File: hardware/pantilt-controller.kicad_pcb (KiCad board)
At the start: 4 copper layers, 52.3 x 93.2 mm, 84 parts, among them J1 Conn_01x22_Socket, J17 Motor_Slide, J18 Motor_Pan, J19 Motor_Tilt, J2 Conn_01x22_Socket, J20 TCA9548A_Mux, J21 AS5600_Pan, J22 AS5600_Tilt, J23 OLED, J24 TCA9548A_Mux, J26 Limit_Min, J27 Limit_Max, J28 Motor_Aux, J29 Enc_Slide, J3 MUX_2, J30 Enc_Pan, J31 Enc_Tilt, J32 Enc_Aux, J33 Btn_SetKeyframe, J34 Btn_ClearKeyframe, J35 Btn_PlayPause, J36 Btn_Reset, J37 5V_In, J38 24V_In, J4 MUX_3, J41 Aux_Max, J5 MUX_4, J6 MUX_5, J7 MUX_6, J8 MUX_7, U1 tmc2209, U2 tmc2209, U3 tmc2209, U4 tmc2209

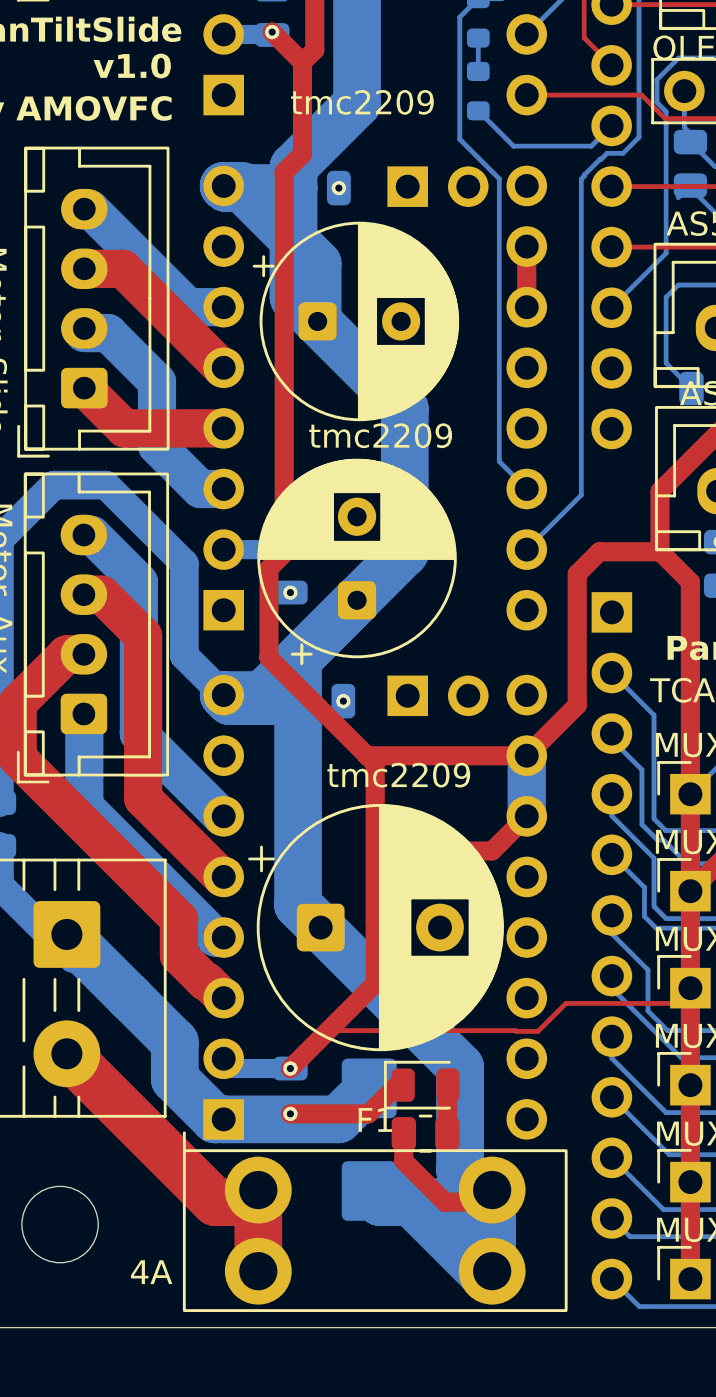
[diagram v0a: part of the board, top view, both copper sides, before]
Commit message: fixes
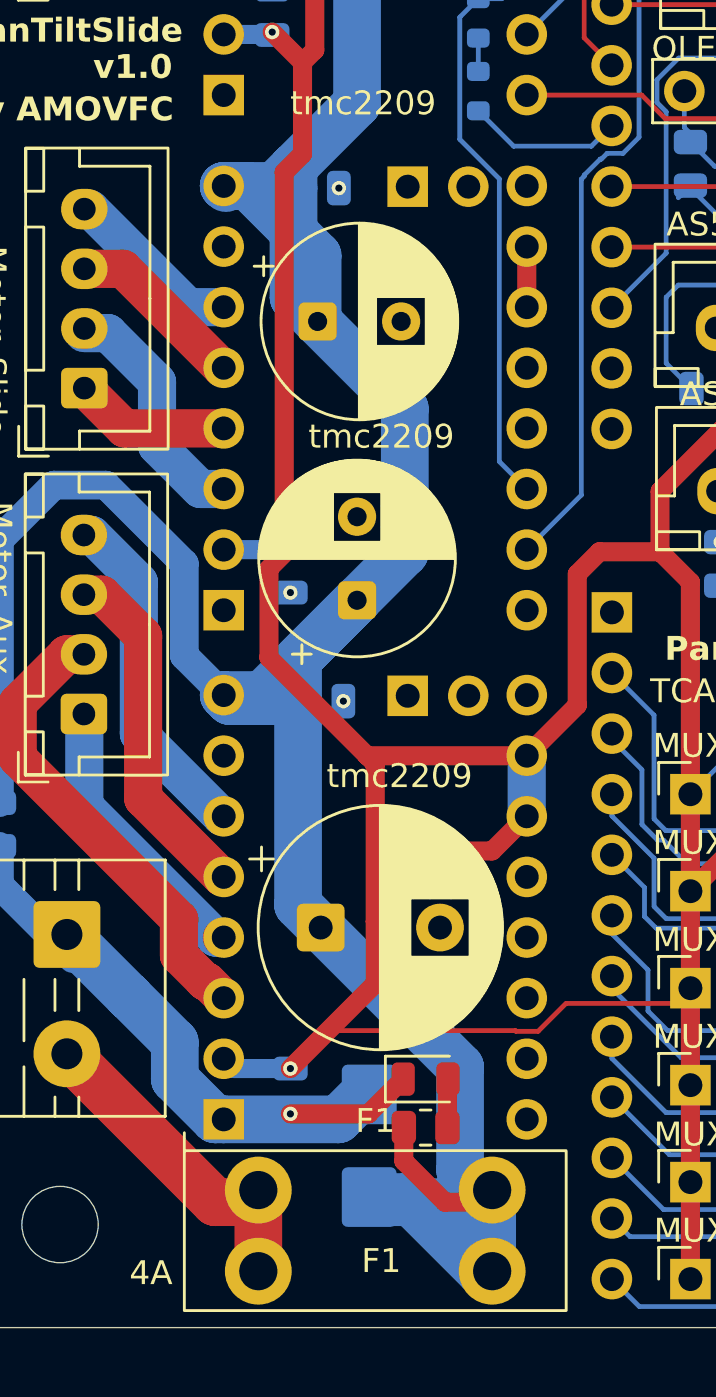
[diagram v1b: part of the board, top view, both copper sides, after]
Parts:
- moved D1 0.25 mm to (104.4, 103.4)
- moved R31 0.25 mm to (106.8, 102.6)
- moved LED1 0.25 mm to (106.8, 100.6)
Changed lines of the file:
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@@
 	(footprint "Resistor_SMD:R_0805_2012Metric"
 		(layer "F.Cu")
-		(at 106.7585 102.87 180)
+		(at 106.7585 102.616 180)
 		(descr "Resistor SMD 0805 (2012 Metric), square (rectangular) end terminal, IPC-7351 nominal, (Body size source: IPC-SM-782 page 72, https://www.pcb-3d.com/wordpress/wp-content/uploads/ipc-sm-782a_amendment_1_and_2.pdf)")
 		(tags "resistor")
@@
 		)
 		(fp_text user "${REFERENCE}"
-			(at 0 0 0)
-			(layer "F.Fab")
+			(at 0.254 1.27 0)
+			(layer "F.SilkS")
 			(effects
 				(font
@@
 	(footprint "LED_SMD:LED_0805_2012Metric"
 		(layer "F.Cu")
-		(at 106.7585 100.838)
+		(at 106.7585 100.584)
 		(descr "LED SMD 0805 (2012 Metric), square (rectangular) end terminal, IPC-7351 nominal, (Body size source: https://docs.google.com/spreadsheets/d/1BsfQQcO9C6DZCsRaXUlFlo91Tg2WpOkGARC1WS5S8t0/edit?usp=sharing)")
 		(tags "LED")
@@
 	(footprint "Diode_SMD:D_SMB"
 		(layer "B.Cu")
-		(at 104.394 103.124 -90)
+		(at 104.394 103.378 -90)
 		(descr "Diode SMB (DO-214AA)")
 		(tags "Diode SMB (DO-214AA)")
@@
 	)
 	(segment
-		(start 137.668 76.7865)
-		(end 137.668 73.66)
+		(start 105.821 100.584)
+		(end 104.363 102.042)
 		(width 0.8)
 		(layer "F.Cu")
@@
 	)
 	(segment
-		(start 105.821 100.584)
-		(end 104.363 102.042)
+		(start 137.668 76.7865)
+		(end 137.668 73.66)
 		(width 0.8)
 		(layer "F.Cu")
@@
 	)
 	(segment
-		(start 103.096094 102.271906)
-		(end 104.394 100.974)
-		(width 2)
-		(layer "B.Cu")
-		(net "GND")
-	)
-	(segment
 		(start 132.2415 86.9425)
 		(end 133.35 85.834)
@@
 	)
 	(segment
+		(start 103.096094 102.271906)
+		(end 104.14 101.228)
+		(width 2)
+		(layer "B.Cu")
+		(net "GND")
+	)
+	(segment
 		(start 88.9 92.4595)
 		(end 91.9805 95.54)
@@
 	)
 	(segment
-		(start 98.298 102.271906)
-		(end 103.096094 102.271906)
+		(start 104.14 101.228)
+		(end 104.394 101.228)
 		(width 2)
 		(layer "B.Cu")
@@
 	)
 	(segment
+		(start 98.298 102.271906)
+		(end 103.096094 102.271906)
+		(width 2)
+		(layer "B.Cu")
+		(net "GND")
+	)
+	(segment
 		(start 98.527906 102.042)
 		(end 98.298 102.271906)
@@
 	)
 	(segment
-		(start 105.846 104.019898)
-		(end 105.846 102.87)
+		(start 107.568102 105.742)
+		(end 105.846 104.019898)
 		(width 0.8)
 		(layer "F.Cu")
@@
 	)
 	(segment
-		(start 107.568102 105.742)
-		(end 105.846 104.019898)
+		(start 105.846 104.019898)
+		(end 105.846 102.616)
 		(width 0.8)
 		(layer "F.Cu")
@@
 	)
 	(segment
-		(start 105.68 105.274)
-		(end 109.04 108.634)
+		(start 98.298 20.066)
+		(end 100.97 20.066)
 		(width 2)
 		(layer "B.Cu")
@@
 	)
 	(segment
-		(start 98.298 20.066)
-		(end 100.97 20.066)
+		(start 105.886 72.486651)
+		(end 102.233349 68.834)
 		(width 2)
 		(layer "B.Cu")
@@
 	)
 	(segment
-		(start 105.886 72.486651)
-		(end 102.233349 68.834)
+		(start 102.233349 68.834)
+		(end 102.233349 66.075254)
 		(width 2)
 		(layer "B.Cu")
@@
 	)
 	(segment
-		(start 98.969905 63.155905)
-		(end 98.298 63.155905)
+		(start 102.233349 66.075254)
+		(end 99.314 63.155905)
 		(width 2)
 		(layer "B.Cu")
@@
 	)
 	(segment
-		(start 102.233349 66.419349)
-		(end 98.969905 63.155905)
+		(start 109.548 105.742)
+		(end 104.862 105.742)
 		(width 2)
 		(layer "B.Cu")
@@
 	)
 	(segment
-		(start 108.204 104.398)
-		(end 108.204 100.076)
-		(width 2)
-		(layer "B.Cu")
-		(net "+24V")
-	)
-	(segment
 		(start 102.233349 47.498)
 		(end 101.412 46.676651)
@@
 	)
 	(segment
+		(start 109.04 108.634)
+		(end 109.548 108.634)
+		(width 2)
+		(layer "B.Cu")
+		(net "+24V")
+	)
+	(segment
 		(start 101.412 84.745906)
 		(end 101.412 82.992)
@@
 	)
 	(segment
-		(start 109.548 105.742)
-		(end 108.204 104.398)
+		(start 100.97 20.066)
+		(end 100.97 24.390651)
 		(width 2)
 		(layer "B.Cu")
@@
 	)
 	(segment
-		(start 100.97 20.066)
-		(end 100.97 24.390651)
+		(start 105.934 105.528)
+		(end 109.04 108.634)
+		(width 2)
+		(layer "B.Cu")
+		(net "+24V")
+	)
+	(segment
+		(start 108.204 100.076)
+		(end 108.204 104.398)
 		(width 2)
 		(layer "B.Cu")
@@
 	)
 	(segment
+		(start 102.362 94.234)
+		(end 108.204 100.076)
+		(width 2)
+		(layer "B.Cu")
+		(net "+24V")
+	)
+	(segment
 		(start 98.388095 41.656)
 		(end 98.298 41.565905)
@@
 	)
 	(segment
-		(start 104.394 105.274)
-		(end 105.68 105.274)
+		(start 98.298 63.155905)
+		(end 100.431557 63.155905)
 		(width 2)
 		(layer "B.Cu")
@@
 	)
 	(segment
-		(start 109.04 108.634)
-		(end 109.548 108.634)
+		(start 99.314 63.155905)
+		(end 98.298 63.155905)
 		(width 2)
 		(layer "B.Cu")
@@
 	)
 	(segment
-		(start 104.862 105.742)
-		(end 104.394 105.274)
-		(width 2)
-		(layer "B.Cu")
-		(net "+24V")
-	)
-	(segment
-		(start 109.548 105.742)
-		(end 104.862 105.742)
+		(start 101.224 63.246)
+		(end 101.224 67.824651)
 		(width 2)
 		(layer "B.Cu")
@@
 	)
 	(segment
-		(start 101.224 63.246)
-		(end 101.224 67.824651)
+		(start 99.035905 41.565905)
+		(end 102.233349 44.763349)
 		(width 2)
 		(layer "B.Cu")
@@
 	)
 	(segment
-		(start 99.035905 41.565905)
-		(end 102.233349 44.763349)
+		(start 103.886 59.701462)
+		(end 101.224 62.363462)
 		(width 2)
 		(layer "B.Cu")
@@
 	)
 	(segment
-		(start 102.233349 68.834)
-		(end 102.233349 66.419349)
+		(start 101.412 46.676651)
+		(end 101.412 41.656)
 		(width 2)
 		(layer "B.Cu")
@@
 	)
 	(segment
-		(start 103.886 59.701462)
-		(end 101.224 62.363462)
+		(start 101.412 84.745906)
+		(end 98.552 84.745906)
 		(width 2)
 		(layer "B.Cu")
@@
 	)
 	(segment
-		(start 98.298 63.155905)
-		(end 99.095254 63.155905)
+		(start 101.979349 22.545268)
+		(end 99.500081 20.066)
 		(width 2)
 		(layer "B.Cu")
@@
 	)
 	(segment
-		(start 101.412 46.676651)
-		(end 101.412 41.656)
+		(start 103.886 80.518)
+		(end 105.886 78.518)
 		(width 2)
 		(layer "B.Cu")
@@
 	)
 	(segment
-		(start 101.412 84.745906)
-		(end 98.552 84.745906)
+		(start 104.648 105.528)
+		(end 104.394 105.528)
 		(width 2)
 		(layer "B.Cu")
@@
 	)
 	(segment
-		(start 101.979349 22.545268)
-		(end 99.500081 20.066)
+		(start 100.431557 63.155905)
+		(end 101.224 62.363462)
 		(width 2)
 		(layer "B.Cu")
@@
 	)
 	(segment
-		(start 103.886 80.518)
-		(end 105.886 78.518)
+		(start 104.862 105.742)
+		(end 104.648 105.528)
 		(width 2)
 		(layer "B.Cu")
@@
 	)
 	(segment
+		(start 108.204 104.398)
+		(end 109.548 105.742)
+		(width 2)
+		(layer "B.Cu")
+		(net "+24V")
+	)
+	(segment
 		(start 96.648 82.841906)
 		(end 96.648 78.980963)
@@
 	)
 	(segment
-		(start 108.204 100.076)
-		(end 102.362 94.234)
-		(width 2)
-		(layer "B.Cu")
-		(net "+24V")
-	)
-	(segment
 		(start 99.912094 84.491906)
 		(end 98.298 84.491906)
@@
 	)
 	(segment
-		(start 101.412 41.656)
-		(end 98.388095 41.656)
+		(start 104.394 105.528)
+		(end 105.934 105.528)
 		(width 2)
 		(layer "B.Cu")
@@
 	)
 	(segment
-		(start 101.224 63.246)
-		(end 98.388095 63.246)
+		(start 101.412 41.656)
+		(end 98.388095 41.656)
 		(width 2)
 		(layer "B.Cu")
@@
 		(start 107.671 100.609)
 		(end 107.696 100.584)
-		(width 0.2)
+		(width 0.8)
 		(layer "F.Cu")
 		(net "Net-(LED1-A)")
 	)
 	(segment
-		(start 107.671 102.6)
+		(start 107.671 102.616)
 		(end 107.671 100.609)
 		(width 0.8)

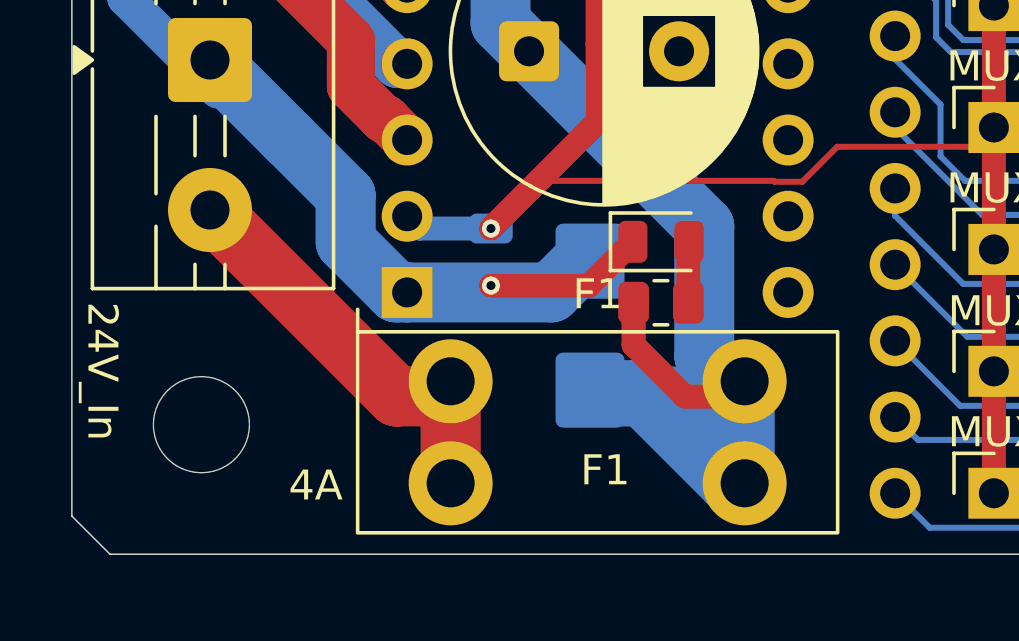
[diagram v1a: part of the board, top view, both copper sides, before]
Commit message: fixing f1
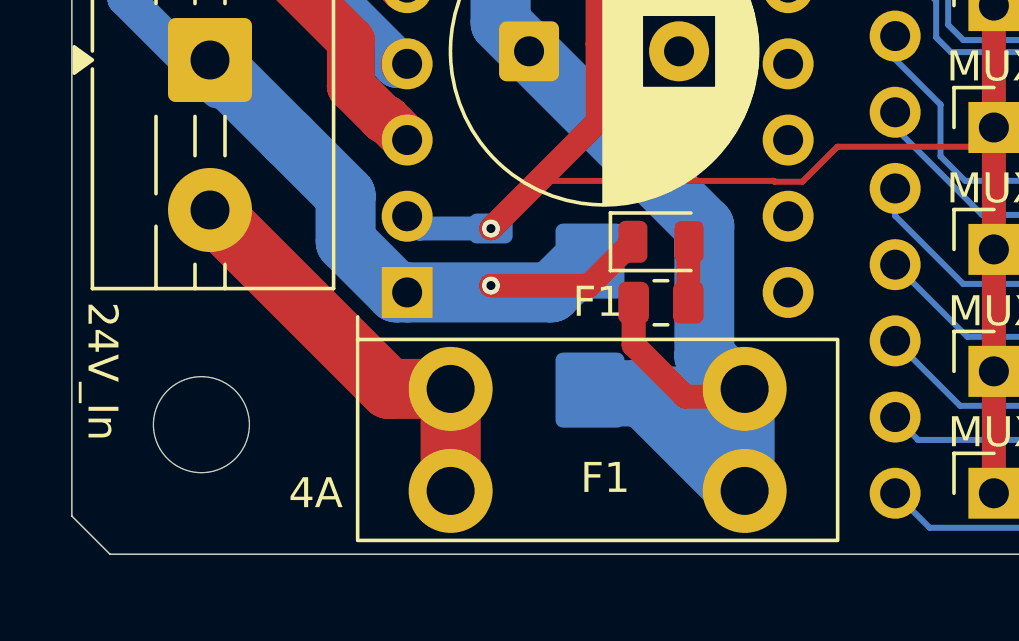
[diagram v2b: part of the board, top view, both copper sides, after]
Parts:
- moved F1 0.25 mm to (104.6, 107.2)
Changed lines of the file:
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@@
 	(footprint "PanTilt:Fuseholder_Blade_Mini_XFCN_XF-508P-B-B"
 		(layer "F.Cu")
-		(at 104.648 106.934)
+		(at 104.648 107.188)
 		(descr "XFCN XF-508P-B-B MINI (ATM) automotive blade fuse holder, THT. Hole grid 9.80 x 3.40mm, 4x 1.6mm min round. Body 16.00 x 6.70mm, 7.35mm tall. 500V, 15-30A. LCSC C19727305.")
 		(tags "fuse holder blade mini ATM automotive XFCN")
@@
 	)
 	(segment
+		(start 109.294 108.634)
+		(end 109.548 108.888)
+		(width 2)
+		(layer "B.Cu")
+		(net "+24V")
+	)
+	(segment
 		(start 102.233349 47.498)
 		(end 101.412 46.676651)
@@
 	)
 	(segment
-		(start 109.04 108.634)
-		(end 109.548 108.634)
-		(width 2)
-		(layer "B.Cu")
-		(net "+24V")
-	)
-	(segment
 		(start 101.412 84.745906)
 		(end 101.412 82.992)
@@
 	)
 	(segment
-		(start 105.934 105.528)
-		(end 109.04 108.634)
+		(start 108.204 100.076)
+		(end 108.204 104.398)
 		(width 2)
 		(layer "B.Cu")
@@
 	)
 	(segment
-		(start 108.204 100.076)
-		(end 108.204 104.398)
+		(start 101.979349 25.4)
+		(end 104.062 27.482651)
 		(width 2)
 		(layer "B.Cu")
@@
 	)
 	(segment
-		(start 101.979349 25.4)
-		(end 104.062 27.482651)
+		(start 105.934 105.528)
+		(end 109.04 108.634)
 		(width 2)
 		(layer "B.Cu")
@@
 	)
 	(segment
+		(start 104.394 105.528)
+		(end 105.934 105.528)
+		(width 2)
+		(layer "B.Cu")
+		(net "+24V")
+	)
+	(segment
 		(start 98.298 84.491906)
 		(end 96.648 82.841906)
@@
 	)
 	(segment
-		(start 109.548 108.634)
-		(end 109.548 105.234)
-		(width 2)
-		(layer "B.Cu")
-		(net "+24V")
-	)
-	(segment
 		(start 99.314 63.155905)
 		(end 98.298 63.155905)
@@
 	)
 	(segment
+		(start 109.04 108.634)
+		(end 109.294 108.634)
+		(width 2)
+		(layer "B.Cu")
+		(net "+24V")
+	)
+	(segment
 		(start 101.979349 25.4)
 		(end 101.979349 22.545268)
@@
 	)
 	(segment
+		(start 109.548 108.888)
+		(end 109.548 105.488)
+		(width 2)
+		(layer "B.Cu")
+		(net "+24V")
+	)
+	(segment
 		(start 102.233349 44.763349)
 		(end 102.233349 47.498)
@@
 	)
 	(segment
-		(start 104.394 105.528)
-		(end 105.934 105.528)
-		(width 2)
-		(layer "B.Cu")
-		(net "+24V")
-	)
-	(segment
 		(start 101.412 41.656)
 		(end 98.388095 41.656)
@@
 	)
 	(segment
-		(start 99.748 105.234)
-		(end 99.748 108.634)
-		(width 2)
-		(layer "F.Cu")
-		(net "Net-(J38-Pin_2)")
-	)
-	(segment
 		(start 91.7265 99.524)
-		(end 97.9445 105.742)
+		(end 97.6905 105.488)
 		(width 2)
 		(layer "F.Cu")
@@
 	)
 	(segment
-		(start 97.9445 105.742)
-		(end 99.24 105.742)
+		(start 99.748 105.488)
+		(end 99.748 108.888)
 		(width 2)
 		(layer "F.Cu")
@@
 	)
 	(segment
-		(start 99.24 105.742)
-		(end 99.748 105.234)
+		(start 97.6905 105.488)
+		(end 99.748 105.488)
 		(width 2)
 		(layer "F.Cu")
